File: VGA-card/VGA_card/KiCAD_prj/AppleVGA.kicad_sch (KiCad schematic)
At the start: 32 parts, among them J1 AppleIIBus, J2 VGA, Q1 DMG2305UX-7, SW1 Reset, U1 74LVC245, U2 74LVC245, U3 74LVC245, U4 74LVC245, U6 Pico

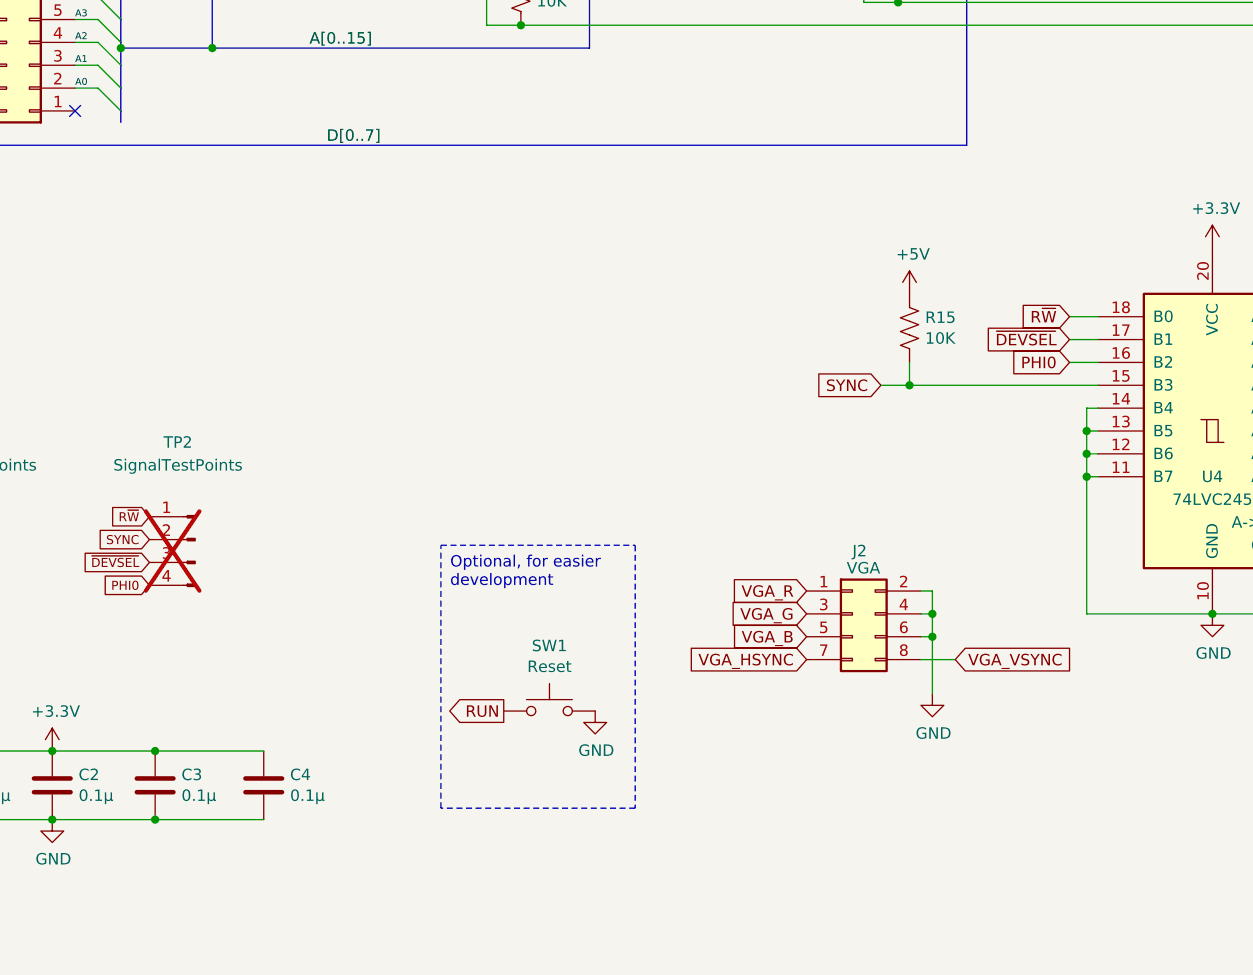
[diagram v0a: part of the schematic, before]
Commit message: VGA card KiCAD project updated
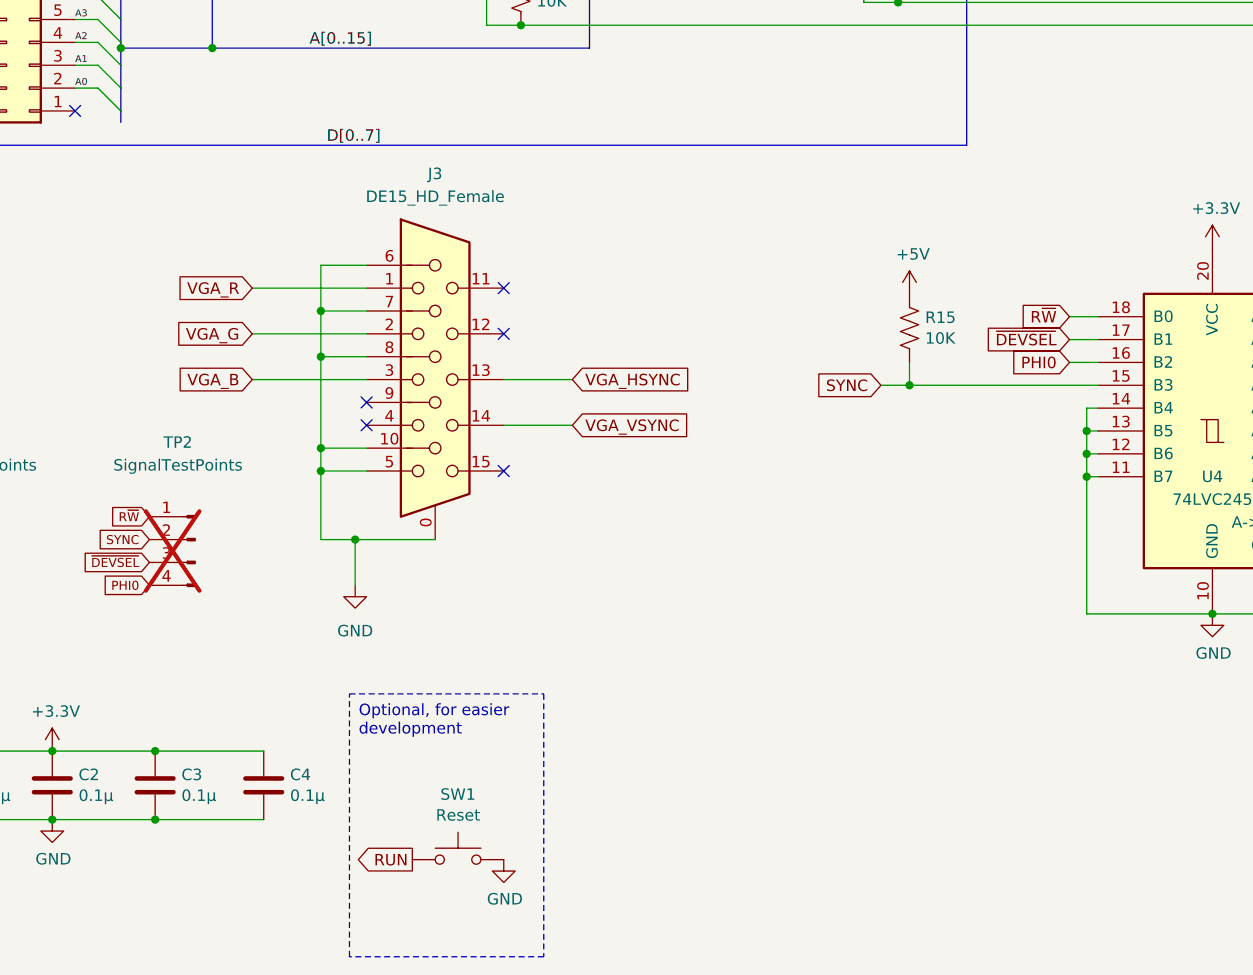
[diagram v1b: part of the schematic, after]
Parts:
- removed J2: VGA, Connector_IDC:IDC-Header_2x04_P2.54mm_Vertical, symbol Connector_Generic:Conn_02x04_Odd_Even
- added J3: DE15_HD_Female, Connector_Dsub:DSUB-15-HD_Female_Horizontal_P2.29x1.98mm_EdgePinOffset8.35mm_Housed_MountingHolesOffset10.89mm, symbol Connector:DE15_Receptacle_HighDensity_MountingHoles
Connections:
- net GND: now also J3.0, J3.10, J3.5, J3.6, J3.7, J3.8
- net VGA_B: now also J3.3
- net VGA_G: now also J3.2
- net VGA_HSYNC: now also J3.13
- net VGA_R: now also J3.1
- net VGA_VSYNC: now also J3.14
- no-connect marks 24 -> 29
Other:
- moved on the sheet: SW1
